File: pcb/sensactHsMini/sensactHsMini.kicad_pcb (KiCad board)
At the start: 2 copper layers, 100 x 86 mm, 84 parts, among them P1 CONN_01X10, P2 CONN_01X08, P3 CONN_01X10, P4 CONN_01X08, P5 CONN_01X01, P6 CONN_01X03, P7 CONN_01X05, P8 CONN_01X02, SW1 SWITCH, U1 STM32F407VETx, U2 HR911105A, U3 KSZ8051, U4 SN65HVD230, U5 LMR14006, U6 DS2482, U7 DFPlayerMini, U8 LM2596Board, U9 LM2596Board, Y1 8MHz, Y2 25MHz

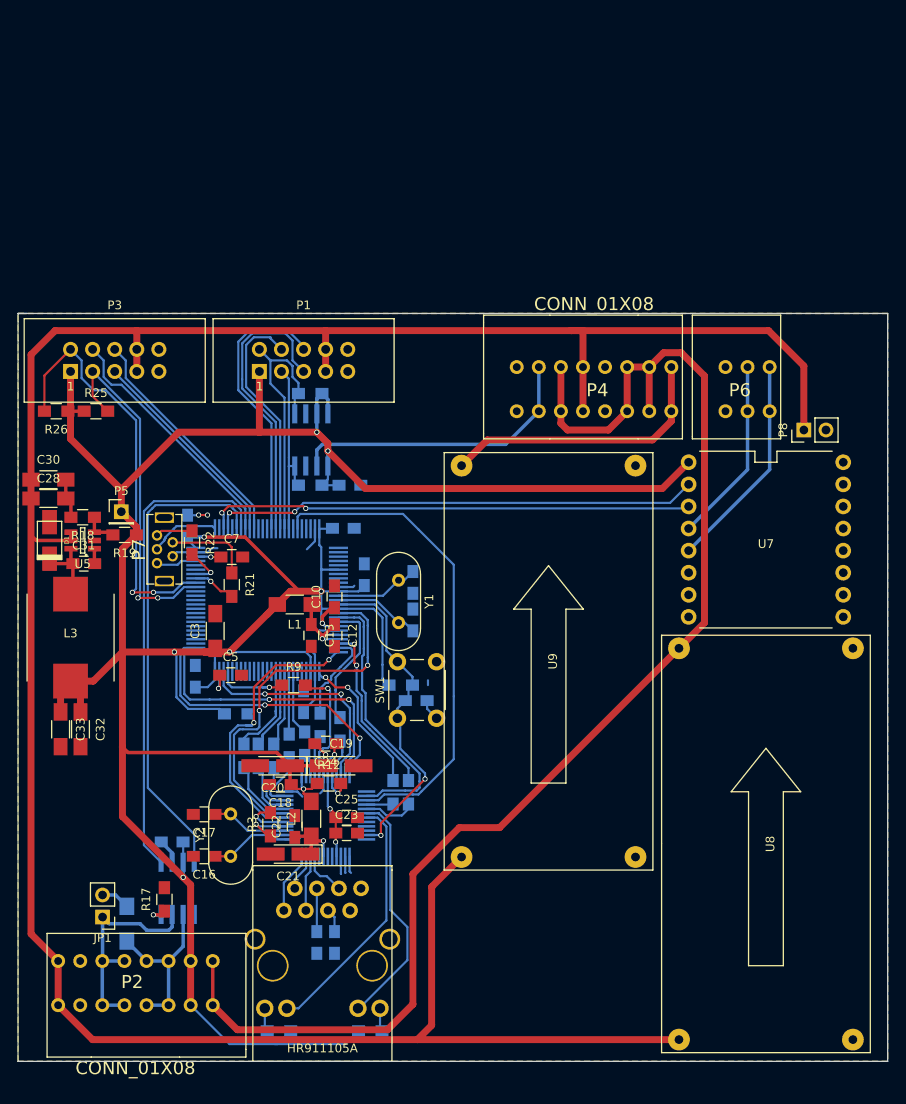
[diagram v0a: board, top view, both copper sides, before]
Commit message: sesnactHsMini &  RPi Hat
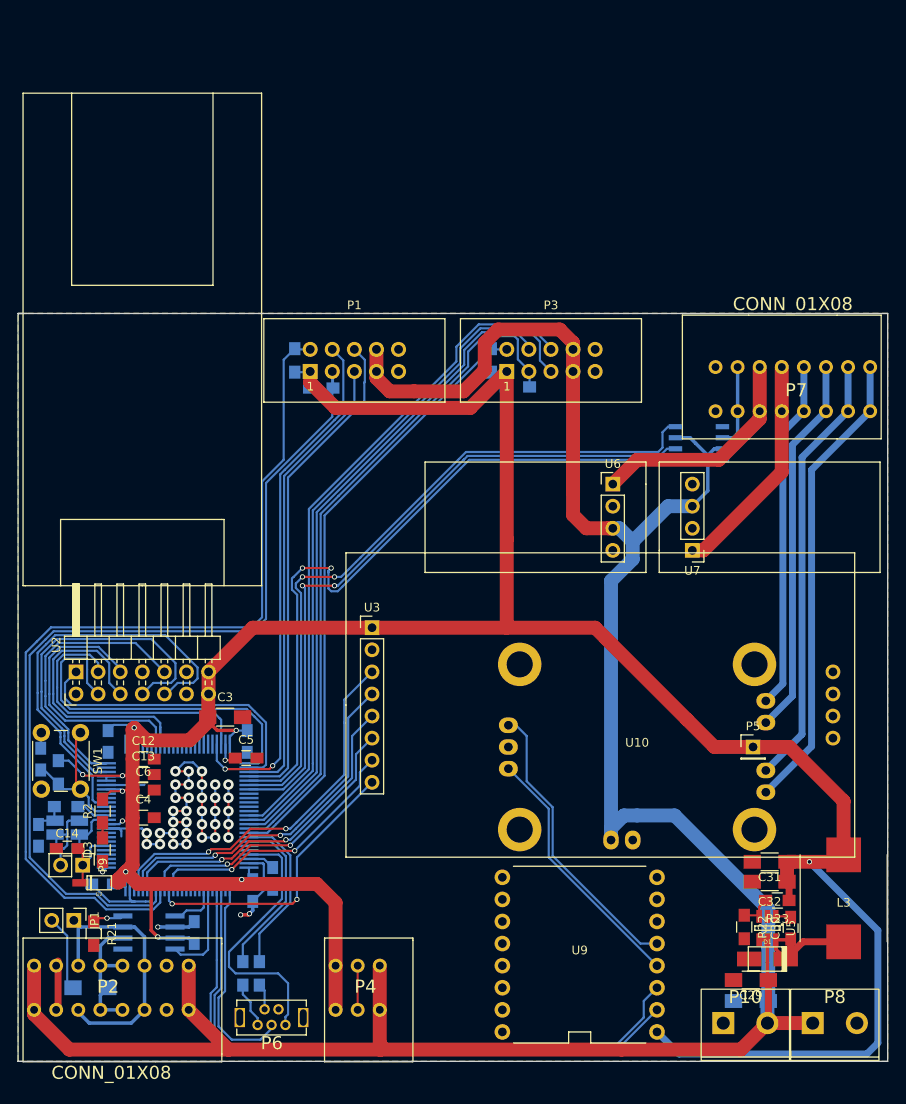
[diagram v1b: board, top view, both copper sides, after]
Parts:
- removed C15, C18, C22, C24, C25: u1, Capacitors_SMD:C_0805_HandSoldering
- removed C16, C17: 22p, Capacitors_SMD:C_0805_HandSoldering
- removed C19, C21: 22u, Capacitors_Tantalum_SMD:CP_Tantalum_Case-A_EIA-3216-18_Hand
- removed C20: 47u, Capacitors_Tantalum_SMD:CP_Tantalum_Case-A_EIA-3216-18_Hand
- removed C23: 2u2, Capacitors_SMD:C_0805_HandSoldering
- removed C33: m1, Capacitors_SMD:C_1206_HandSoldering
- removed L1, L2: Ferrite_Bead, Resistors_SMD:R_1206_HandSoldering
- removed R10, R11, R13, R14, R15, R5, R6, R7, R8, R9: 33R, Resistors_SMD:R_0805_HandSoldering
- removed R12: 4k7, Resistors_SMD:R_0805_HandSoldering
- removed R3: 6k49, Resistors_SMD:R_0805_HandSoldering
- removed R4: 1k, Resistors_SMD:R_0805_HandSoldering
- removed Y2: 25MHz, Crystals:Crystal_HC49-U_Vertical
- added D2: D, sensact:sod123_handsolder, F.Cu at (29.3, 85.5)
- added D3: LED, Resistors_SMD:R_0805_HandSoldering, F.Cu at (29.7, 81.7)
- added P10: 24V_IN, sensact:conn_2P, F.Cu at (103.6, 101.6)
- added P9: BACKUP, Pin_Headers:Pin_Header_Straight_1x02_Pitch2.54mm, F.Cu at (27.4, 83.4)
- added U10: MODULE_TPA3110stereo, sensact:MODULE_TPA3110stereo, F.Cu at (91.2, 69.8)
- C10, C28, C7: moved to B.Cu
- C14, C4, C6: moved to F.Cu
- C29: value C -> 4u7; footprint Capacitors_SMD:C_0805_HandSoldering -> Capacitors_SMD:C_1206_HandSoldering; moved to F.Cu
- C30: value 4u7 -> u15; footprint Capacitors_SMD:C_1206_HandSoldering -> Capacitors_SMD:C_0805_HandSoldering
- C31: value u15 -> 10u; footprint Capacitors_SMD:C_0805_HandSoldering -> Capacitors_SMD:C_1206_HandSoldering
- C32: value 10u -> m1
- P4: value CONN_01X08 -> CONN_01X03; footprint sensact:KF141R-8p -> sensact:KF141R-3p
- P6: value CONN_01X03 -> CONN_01X05; footprint sensact:KF141R-3p -> sensact:miniusb_vert
- P7: value CONN_01X05 -> CONN_01X08; footprint sensact:miniusb_vert -> sensact:KF141R-8p
- P8: value CONN_01X02 -> 24V_OUT; footprint Pin_Headers:Pin_Header_Straight_1x02_Pitch2.54mm -> sensact:conn_2P
- R1: value 220R -> K22
- R17: value 10k -> 4k7; moved to B.Cu
- R18: value 1k -> 4k7; moved to B.Cu
- R19: value 3k3 -> 4k7; moved to B.Cu
- R2: value 220R -> k1; moved to F.Cu
- R20: value 120R -> 4k7; footprint Resistors_SMD:R_1206_HandSoldering -> Resistors_SMD:R_0805_HandSoldering
- R21: value 100R -> 10k
- R22: value 100R -> 1k
- R23: value 4k7 -> 3k3; moved to F.Cu
- R24: value 4k7 -> 120R; footprint Resistors_SMD:R_0805_HandSoldering -> Resistors_SMD:R_1206_HandSoldering
- R25, R26: value 4k7 -> 100R; moved to B.Cu
- U2: value HR911105A -> MODULE_LAN8720; footprint sensact:HR911105A -> sensact:MODULE_LAN8720
- U3: value KSZ8051 -> MODULE_ST7735_1_8; footprint sensact:LQFP-48_7x7mm_Pitch0.5mm_handsolder -> sensact:MODULE_ST7735_18; moved to F.Cu
- U6: value DS2482 -> MODULE_STEPDOWN; footprint sensact:SOIC-8_3.9x4.9mm_Pitch1.27mm_handsolder -> sensact:MODULE_STEPDOWN; moved to F.Cu
- U7: value DFPlayerMini -> MODULE_STEPDOWN; footprint sensact:DFPlayerMini -> sensact:MODULE_STEPDOWN
- U8: value LM2596Board -> TJA1021T; footprint sensact:LM2596Board -> Housings_SOIC:SOIC-8_3.9x4.9mm_Pitch1.27mm; moved to B.Cu
- U9: value LM2596Board -> DFPlayerMini; footprint sensact:LM2596Board -> sensact:DFPlayerMini
- Y1: value 8MHz -> Crystal_GND24; footprint Crystals:Crystal_HC49-U_Vertical -> sensact:quartz3225; moved to B.Cu
- moved C30 99.7 mm to (108.8, 90.7), turned to 90 degrees
- moved C28 99.3 mm to (104.3, 99.1), turned to 180 degrees
- moved D1 95.6 mm to (106.2, 94.2), turned to 0 degrees
- moved L3 93.8 mm to (114.9, 87.2), turned to 0 degrees
- moved U5 90.5 mm to (106.2, 90.7), turned to 270 degrees
- moved P6 89.9 mm to (49.1, 101.0), turned to 0 degrees
- moved C31 86.0 mm to (106.4, 83.1), turned to 180 degrees
- moved C32 81.2 mm to (106.4, 85.3), turned to 180 degrees
- moved P5 77.5 mm to (104.5, 69.8)
- moved R22 77.4 mm to (103.5, 90.6)
- moved R20 77.1 mm to (74.4, 25.4), turned to 90 degrees
- moved P7 74.6 mm to (109.1, 28.7), turned to 180 degrees
- moved P4 73.5 mm to (60.3, 97.5), turned to 0 degrees
- moved C29 73.2 mm to (104.3, 96.6), turned to 180 degrees
- moved R24 72.9 mm to (28.3, 97.5), turned to 0 degrees
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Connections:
- net Net-(C1-Pad1) renamed /STM32F407VET/OSC_IN
- net Net-(C5-Pad1) renamed /STM32F407VET/VCAP1
- net Net-(C7-Pad1) renamed /STM32F407VET/VCAP2
- C12 pad 1: /STM32F407VET/VDDA -> +3V3
- C13 pad 1: /STM32F407VET/VDDA -> +3V3
- C14 pad 1: Net-(C14-Pad1) -> GND
- C14 pad 2: GND -> /STM32F407VET/VBAT
- C2 pad 1: Net-(C2-Pad1) -> /STM32F407VET/OSC_OUT_X
- C29 pad 1: +3V3 -> +24V
- C30 pad 1: +24V -> Net-(C30-Pad1)
- C30 pad 2: GND -> Net-(C30-Pad2)
- C31 pad 1: Net-(C31-Pad1) -> +3V3
- C31 pad 2: Net-(C31-Pad2) -> GND
- D1 pad 2: Net-(C31-Pad1) -> Net-(C30-Pad1)
- L3 pad 2: Net-(C31-Pad1) -> Net-(C30-Pad1)
- P2 pad 4: /other/CANH -> /other/CANL
- P2 pad 6: /other/CANL -> /other/CANH
- P2 pad 7: +3V3 -> GND
- P2 pad 8: +5V -> +24V
- P4 pad 1: +12V -> +3V3
- P4 pad 2: +5V -> GND
- P4 pad 3: +5V -> +24V
- P6 pad 1: Net-(P6-Pad1) -> SWDIO
- P6 pad 2: Net-(P6-Pad2) -> GND
- P6 pad 3: GND -> SWCLK
- P7 pad 1: SWDIO -> AUDIO_R-
- P7 pad 2: GND -> AUDIO_R+
- P7 pad 3: SWCLK -> AUDIO_L-
- P7 pad 4: Net-(P7-Pad4) -> AUDIO_L+
- P7 pad 5: Net-(P7-Pad5) -> +12V
- R1 pad 1: +3V3 -> /STM32F407VET/OSC_OUT
- R1 pad 2: Net-(R1-Pad2) -> /STM32F407VET/OSC_OUT_X
- R16 pad 2: RST -> SDA1
- R17 pad 1: Net-(R17-Pad1) -> +3V3
- R17 pad 2: GND -> RST
- R18 pad 1: Net-(R18-Pad1) -> +3V3
- R18 pad 2: GND -> SCL1
- R19 pad 2: Net-(R18-Pad1) -> SDA2
- R2 pad 1: +3V3 -> Net-(D3-Pad2)
- R2 pad 2: Net-(R2-Pad2) -> +3V3
- R20 pad 1: Net-(JP1-Pad2) -> +3V3
- R20 pad 2: /other/CANL -> SCL2
- R21 pad 1: Net-(P7-Pad4) -> /other/CAN_RS
- R21 pad 2: TX1 -> GND
- R22 pad 1: Net-(P7-Pad5) -> Net-(R22-Pad1)
- R22 pad 2: RX1 -> GND
- R23 pad 2: SDA1 -> Net-(R22-Pad1)
- R24 pad 1: +3V3 -> Net-(JP1-Pad2)
- R24 pad 2: SCL1 -> /other/CANL
- R25 pad 1: +3V3 -> Net-(P6-Pad4)
- R25 pad 2: SDA2 -> TX1
- R26 pad 1: +3V3 -> Net-(P6-Pad5)
- R26 pad 2: SCL2 -> RX1
- U1 pad 1: (no net) -> Net-(D3-Pad1)
- U1 pad 13: Net-(C2-Pad1) -> /STM32F407VET/OSC_OUT
- U1 pad 15: +3V3 -> (no net)
- U1 pad 16: MDC -> ETH_MDC
- U1 pad 17: TXD2 -> (no net)
- U1 pad 18: TXC -> (no net)
- U1 pad 21: /STM32F407VET/VDDA -> +3V3
- U1 pad 22: /STM32F407VET/VDDA -> +3V3
- U1 pad 23: CRS -> ETH_CRS
- U1 pad 24: RXC -> (no net)
- U1 pad 25: MDIO -> ETH_MDIO
- U1 pad 26: COL -> (no net)
- U1 pad 32: RXDV -> (no net)
- U1 pad 33: RXD0 -> ETH_RX0
- U1 pad 34: RXD1 -> ETH_RX1
- U1 pad 35: RXD2 -> (no net)
- U1 pad 36: RXD3 -> (no net)
- U1 pad 47: RXER -> INT1_1
- U1 pad 48: TXEN -> ETH_TXEN
- U1 pad 51: TXD0 -> ETH_TX0
- U1 pad 52: TXD1 -> ETH_TX1
- U1 pad 53: (no net) -> INT1_2
- U1 pad 54: (no net) -> INT1_3
- U1 pad 55: (no net) -> LIN_TX
- U1 pad 56: (no net) -> LIN_RX
- U1 pad 57: (no net) -> LIN_SLP
- U1 pad 6: +3V3 -> /STM32F407VET/VBAT
- U1 pad 63: (no net) -> INT2_3
- U1 pad 64: (no net) -> INT2_2
- U1 pad 65: (no net) -> INT2_1
- U1 pad 83: INT2_1 -> (no net)
- U1 pad 84: INT2_2 -> (no net)
- U1 pad 85: INT2_3 -> (no net)
- U1 pad 89: INT1_3 -> LCD_SCK
- U1 pad 90: INT1_2 -> LCD_LED
- U1 pad 91: INT1_1 -> LCD_MOSI
- U1 pad 94: (no net) -> GND
- U1 pad 95: TXD3 -> LCD_A0
- U1 pad 96: (no net) -> LCD_RESET
- U1 pad 97: (no net) -> LCD_CS
- U2 pad 1: Net-(U2-Pad1) -> ETH_TX1
- U2 pad 10: Net-(U2-Pad10) -> ETH_MDC
- U2 pad 11: Net-(U2-Pad11) -> GND
- U2 pad 12: Net-(R1-Pad2) -> GND
- U2 pad 13: (no net) -> +3V3
- U2 pad 14: (no net) -> +3V3
- U2 pad 2: Net-(U2-Pad2) -> (no net)
- U2 pad 3: Net-(U2-Pad3) -> ETH_TXEN
- U2 pad 4: Net-(C14-Pad1) -> ETH_TX0
- U2 pad 5: Net-(C15-Pad1) -> ETH_RX0
- U2 pad 6: Net-(U2-Pad6) -> ETH_RX1
- U2 pad 8: GND -> ETH_CRS
- U2 pad 9: Net-(R2-Pad2) -> ETH_MDIO
- U3 pad 1: GND -> +3V3
- U3 pad 10: Net-(U2-Pad3) -> (no net)
- U3 pad 11: Net-(U2-Pad2) -> (no net)
- U3 pad 12: Net-(U2-Pad1) -> (no net)
- U3 pad 3: GND -> LCD_CS
- U3 pad 4: +1V2 -> LCD_RESET
- U3 pad 5: (no net) -> LCD_A0
- U3 pad 6: (no net) -> LCD_MOSI
- U3 pad 7: +3.3VA -> LCD_SCK
- U3 pad 8: (no net) -> LCD_LED
- U3 pad 9: Net-(U2-Pad6) -> (no net)
- U4 pad 8: Net-(R17-Pad1) -> /other/CAN_RS
- U5 pad 1: Net-(C31-Pad2) -> Net-(C30-Pad2)
- U5 pad 3: Net-(R18-Pad1) -> Net-(R22-Pad1)
- U5 pad 6: Net-(C31-Pad1) -> Net-(C30-Pad1)
- U6 pad 1: +3V3 -> +5V
- U6 pad 2: /other/1Wa -> GND
- U6 pad 3: GND -> +24V
- U6 pad 4: SDA1 -> (no net)
- U7 pad 1: +3V3 -> +12V
- U7 pad 2: RX2 -> GND
- U7 pad 3: TX2 -> +24V
- U7 pad 4: Net-(P6-Pad2) -> (no net)
- U8 pad 1: +24V -> LIN_TX
- U8 pad 2: GND -> LIN_SLP
- U8 pad 3: GND -> +24V
- U8 pad 4: +5V -> LIN_RX
- U9 pad 1: +24V -> +3V3
- U9 pad 2: GND -> RX2
- U9 pad 3: GND -> TX2
- U9 pad 4: +12V -> /other/AUDIO_R
- Y1 pad 2: Net-(C2-Pad1) -> GND
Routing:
- net +5V: track 176.8 -> 26.0 mm
- net SDA1: track 21.7 -> 104.4 mm
- net LIN_TX: track 0.00 -> 81.7 mm, vias 0 -> 2
- net LIN_RX: track 0.00 -> 80.3 mm, vias 0 -> 2
- net LIN_SLP: track 0.00 -> 78.1 mm, vias 0 -> 2
- net SCL1: track 30.6 -> 106.8 mm
- net GND: track 49.4 -> 107.4 mm, vias 3 -> 32
- net TXD3: track 56.3 -> 0.00 mm
- net INT2_2: track 24.5 -> 80.0 mm
- net AUDIO_R-: track 0.00 -> 54.0 mm
- net INT2_3: track 27.3 -> 78.0 mm
- net AUDIO_R+: track 0.00 -> 50.3 mm
- net CANT: track 55.4 -> 6.09 mm
- net ETH_MDC: track 0.00 -> 48.3 mm
- net INT2_1: track 28.6 -> 75.3 mm
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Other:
- net class 24V added: clearance 0.3, trace_width 0.25, via_dia 0.6, via_drill 0.4
